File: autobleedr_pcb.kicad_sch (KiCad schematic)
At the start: 20 parts, among them J1 Barrel_Jack, J10 XT60 Connector, J11 Conn_01x02_Pin, J12 Linear Actuator Screw_Termina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, J2 Conn_01x13_Pin, J3 Conn_01x14_Pin, J4 Conn_01x08_Socket, J5 IR LED, J6 Photo Transistor, J7 Screw_Terminal_01x02, J8 Conn_01x02_Pin, J9 Conn_01x02_Pin

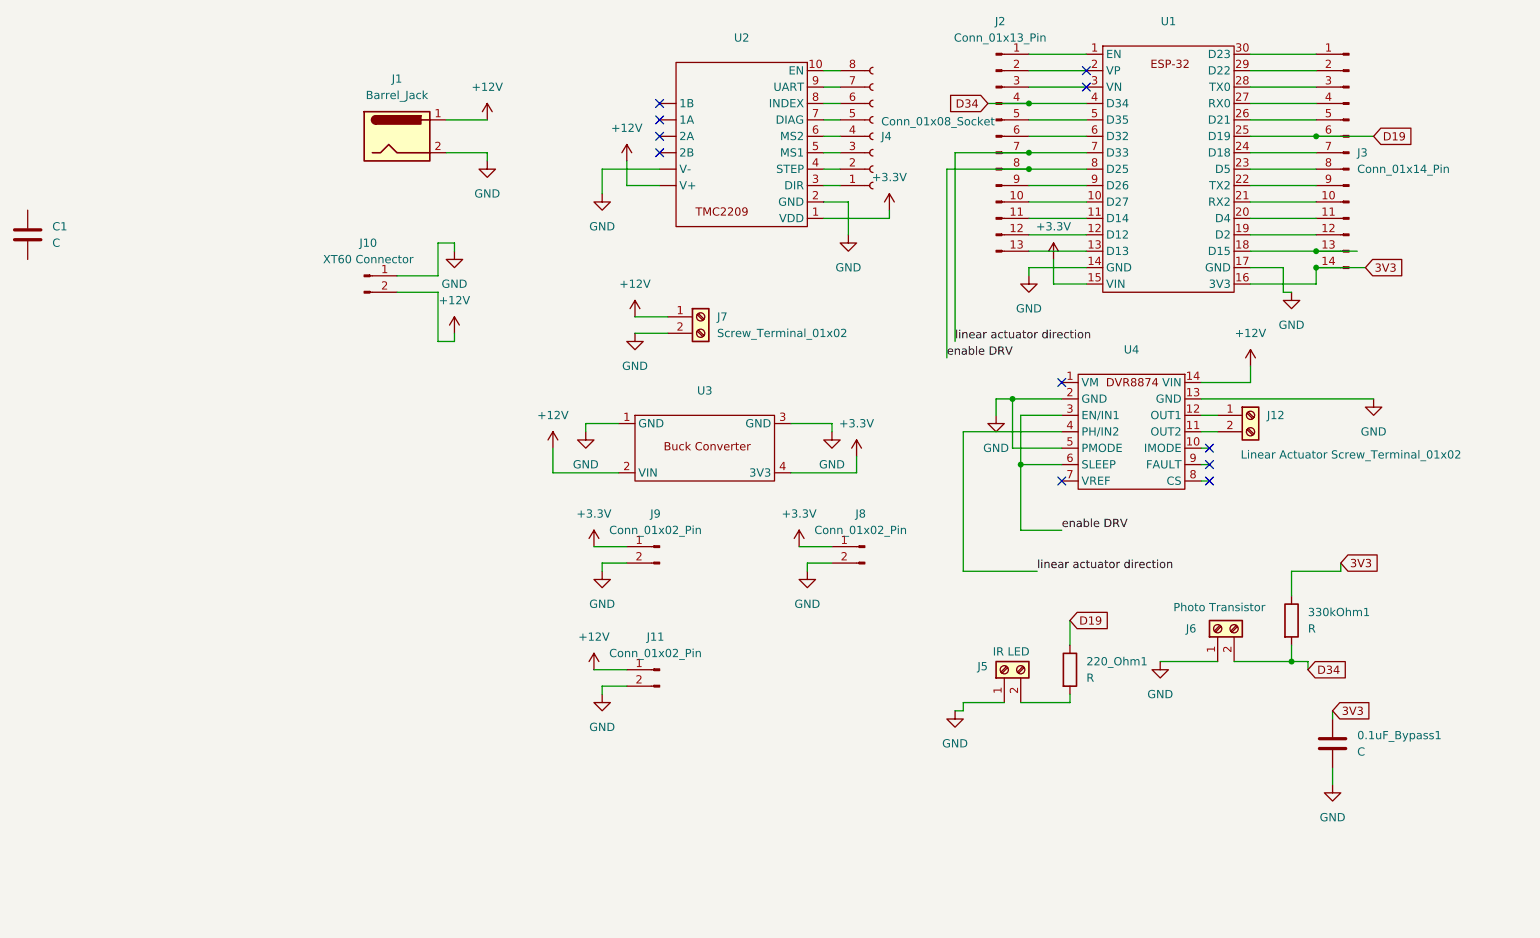
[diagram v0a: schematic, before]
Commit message: updated schematic
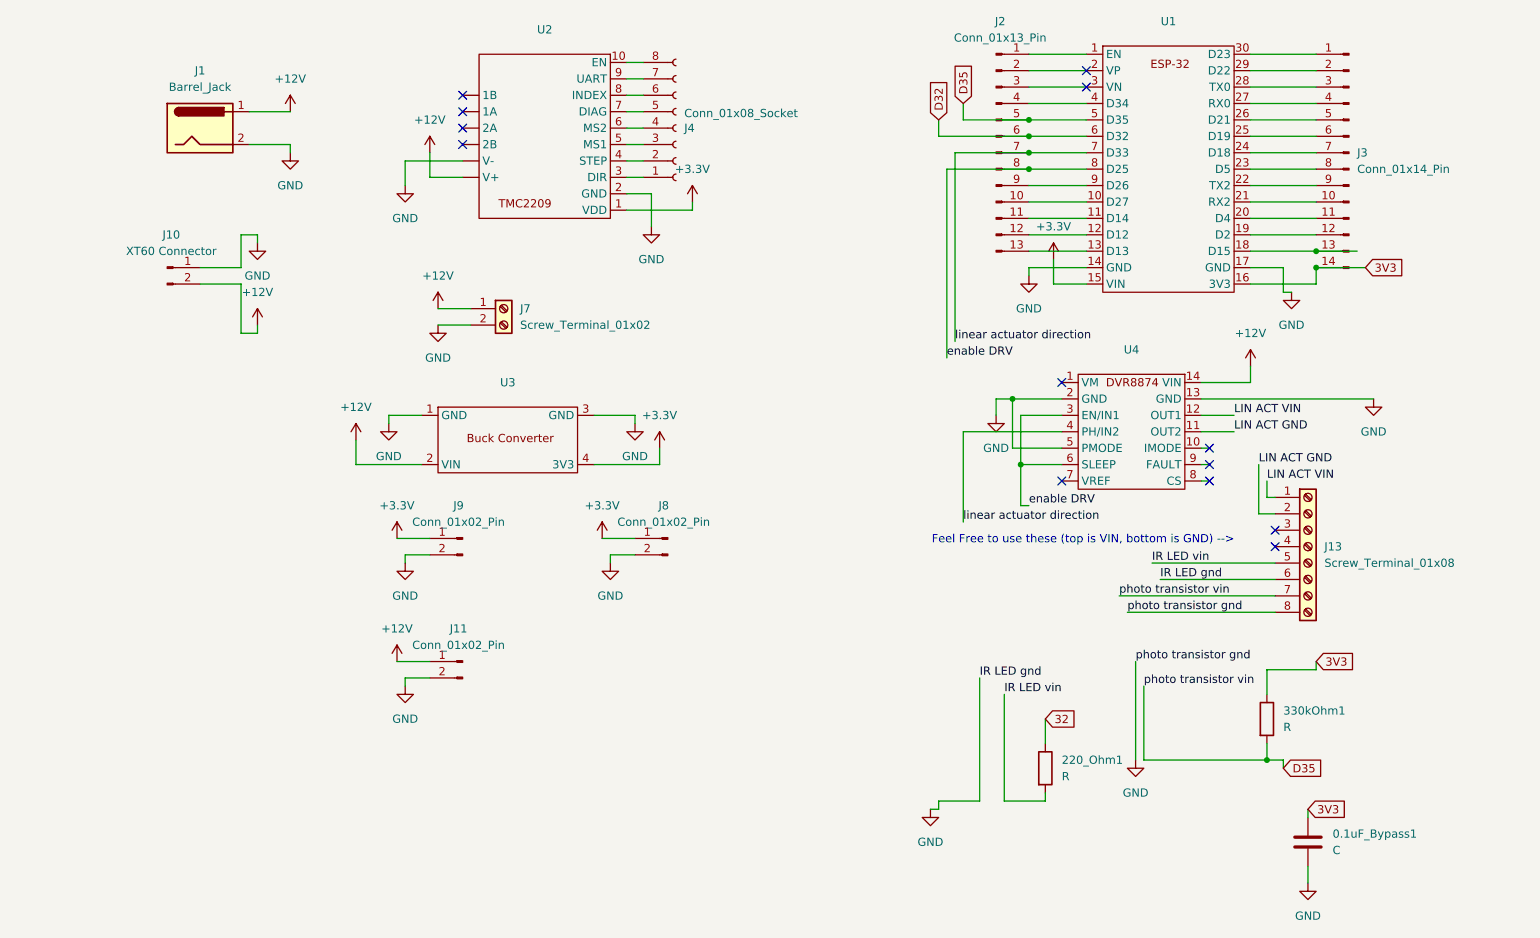
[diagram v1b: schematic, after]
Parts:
- removed C1: C, symbol Device:C
- removed J12: Linear Actuator Screw_Terminal_01x02, TerminalBlock:TerminalBlock_MaiXu_MX126-5.0-02P_1x02_P5.00mm, symbol Connector:Screw_Terminal_01x02
- removed J5: IR LED, TerminalBlock:TerminalBlock_MaiXu_MX126-5.0-02P_1x02_P5.00mm, symbol Connector:Screw_Terminal_01x02
- removed J6: Photo Transistor, TerminalBlock:TerminalBlock_MaiXu_MX126-5.0-02P_1x02_P5.00mm, symbol Connector:Screw_Terminal_01x02
- added J13: Screw_Terminal_01x08, Screw_Terminal_1x8:Screw_Terminal_1x8, symbol Connector:Screw_Terminal_01x08
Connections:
- net GND: now also J13.6 (Pin_6), J13.8 (Pin_8)
- net LIN ACT VIN: now reaches U4.12 (OUT1)
- net LIN ACT VIN: now also J13.1 (Pin_1)
- net LIN ACT GND: now reaches U4.11 (OUT2)
- net LIN ACT GND: now also J13.2 (Pin_2)
- net D35: now reaches J2.5 (Pin_5), U1.5 (D35)
- net D35: now also 330kOhm1.2, J13.7 (Pin_7)
- net D32: now reaches J2.6 (Pin_6), U1.6 (D32)
- net IR LED vin: now reaches 220_Ohm1.2
- net IR LED vin: now also J13.5 (Pin_5)
- net D19: no longer names the net of J3.6 (Pin_6), U1.25 (D19)
- net D19: no longer 220_Ohm1.1
- net D34: no longer names the net of J2.4 (Pin_4), U1.4 (D34)
- net D34: no longer 330kOhm1.2
- new net 32: 220_Ohm1.1
- no-connect marks 11 -> 13
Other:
- note added: "Feel Free to use these (top is VIN, bottom is GND) -->"
- moved on the sheet: 0.1uF_Bypass1, 220_Ohm1, 330kOhm1, J1, J10, J11, J4, J7, J8, J9, U2, U3
